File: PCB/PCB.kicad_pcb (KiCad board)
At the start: 2 copper layers, 110 x 100 mm, 53 parts, among them J1 Conn_01x03, J2 Conn_01x02, Q1 2N2907, Q10 TIP32, Q11 BD138, Q12 TIP31, Q13 2N2222, Q2 2N2907, Q3 2N2907, Q4 2N2222, Q5 2N2222, Q6 2N2907, Q7 2N2907, Q8 BD139, Q9 BD139, U11 Relai, U2 Jack_Mono

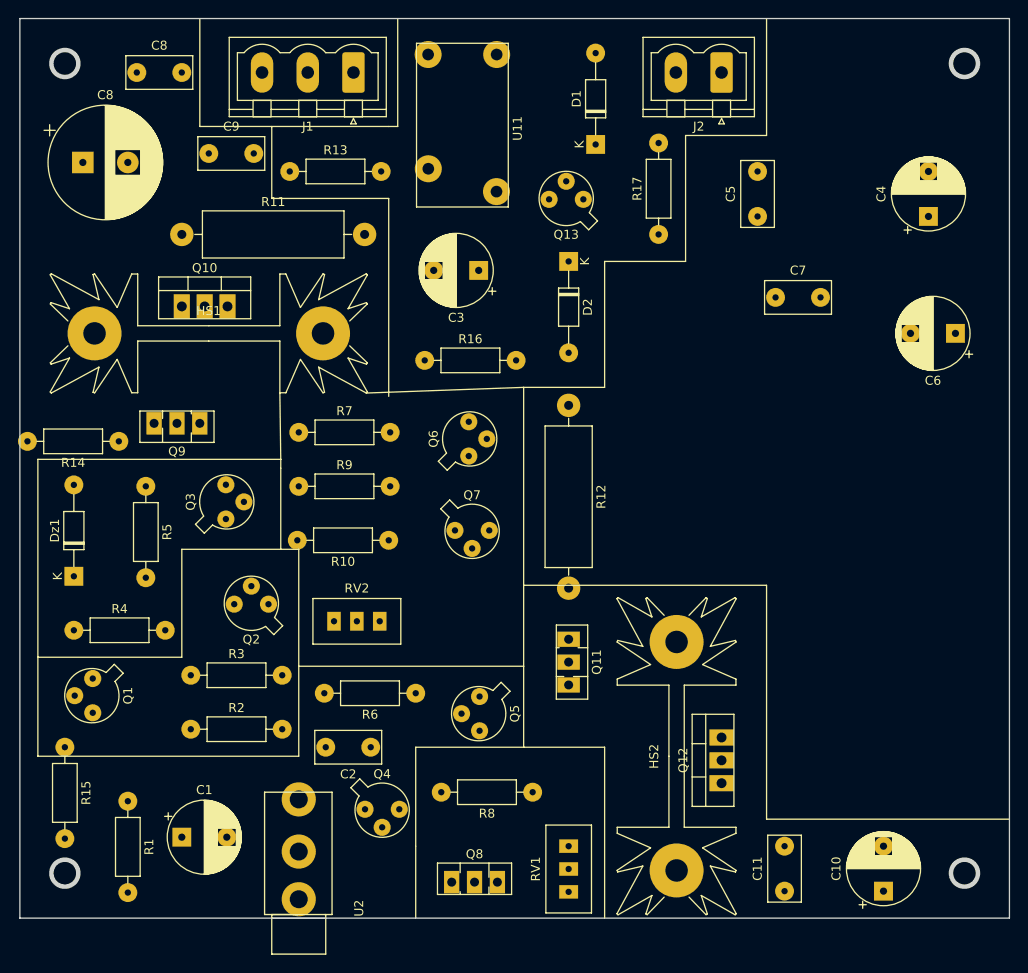
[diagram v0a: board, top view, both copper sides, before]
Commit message: Placmement terminé, demande de go/nogo
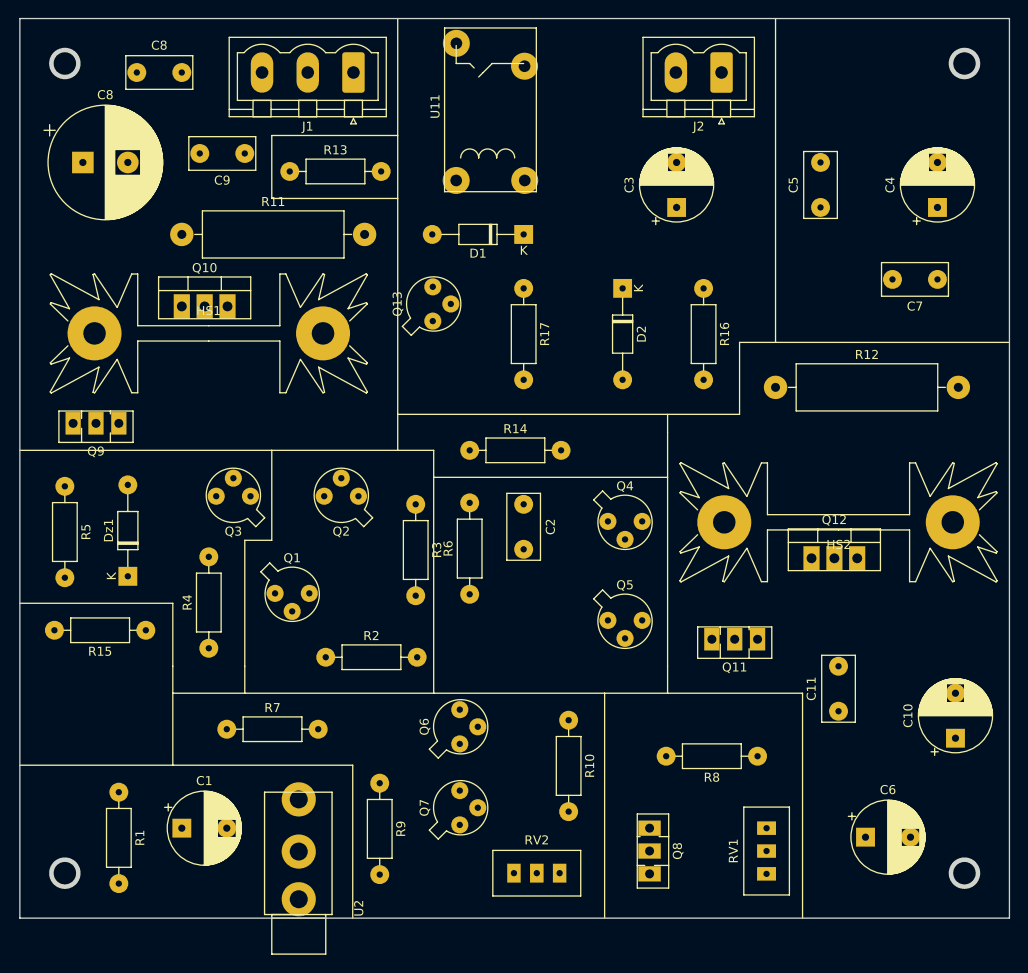
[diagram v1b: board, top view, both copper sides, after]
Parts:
- moved C6 56.9 mm to (134.0, 141.0), turned to 0 degrees
- moved Q4 41.9 mm to (106.0, 106.0)
- moved R14 39.0 mm to (90.0, 98.0), turned to 0 degrees
- moved RV2 34.4 mm to (100.0, 145.0)
- moved R9 34.2 mm to (80.0, 135.0), turned to 270 degrees
- moved R7 34.0 mm to (63.0, 129.0)
- moved Q6 32.0 mm to (89.0, 130.0)
- moved R16 32.0 mm to (116.0, 80.0), turned to 270 degrees
- moved Q7 32.0 mm to (89.0, 139.0), turned to 90 degrees
- moved C2 31.9 mm to (96.0, 104.0), turned to 270 degrees
- moved HS2 31.6 mm to (131.0, 106.0), turned to 180 degrees
- moved R3 31.4 mm to (84.0, 104.0), turned to 270 degrees
- moved R10 28.3 mm to (101.0, 128.0), turned to 270 degrees
- moved Q12 26.9 mm to (128.0, 110.0), turned to 0 degrees
- moved R8 25.3 mm to (122.0, 132.0)
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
